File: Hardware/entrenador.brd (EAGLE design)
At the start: 121.9 x 70.8 mm, 68 parts, among them U1 DRV8833

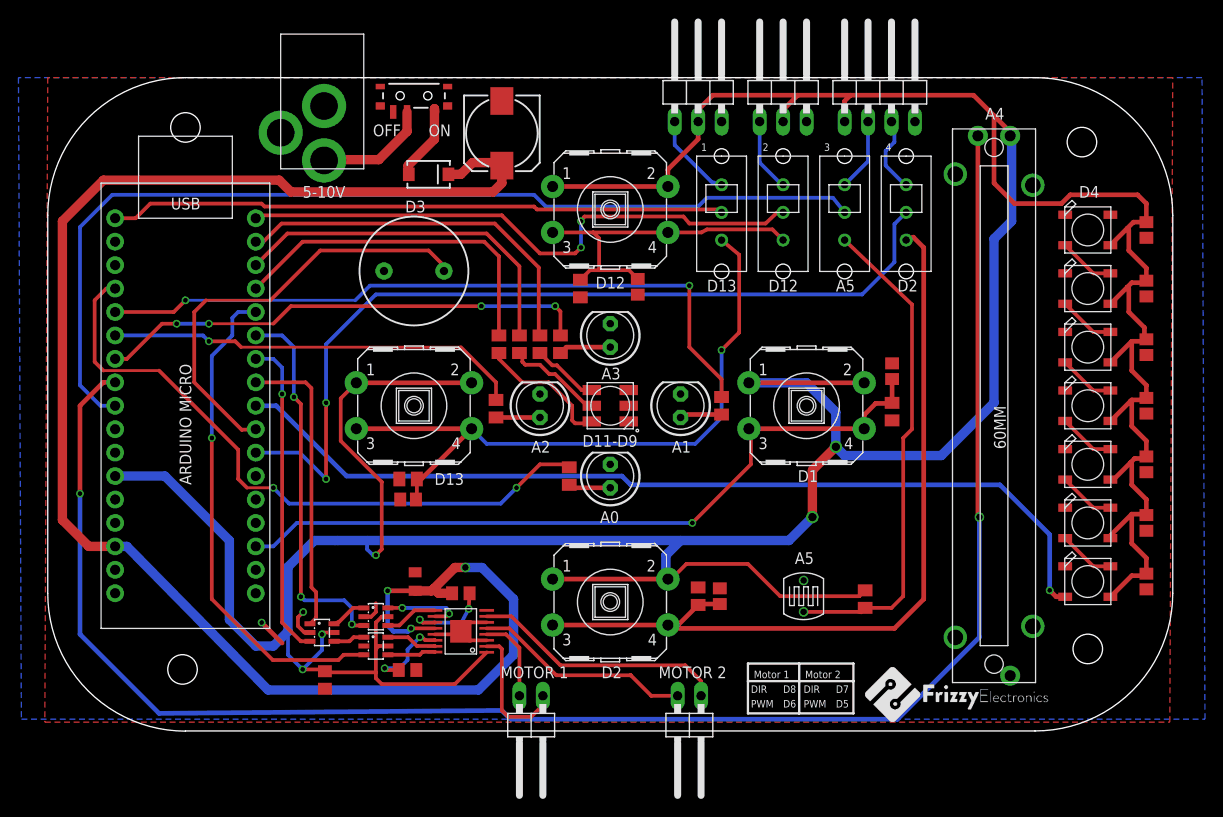
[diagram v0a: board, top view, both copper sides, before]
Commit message: Ultima version
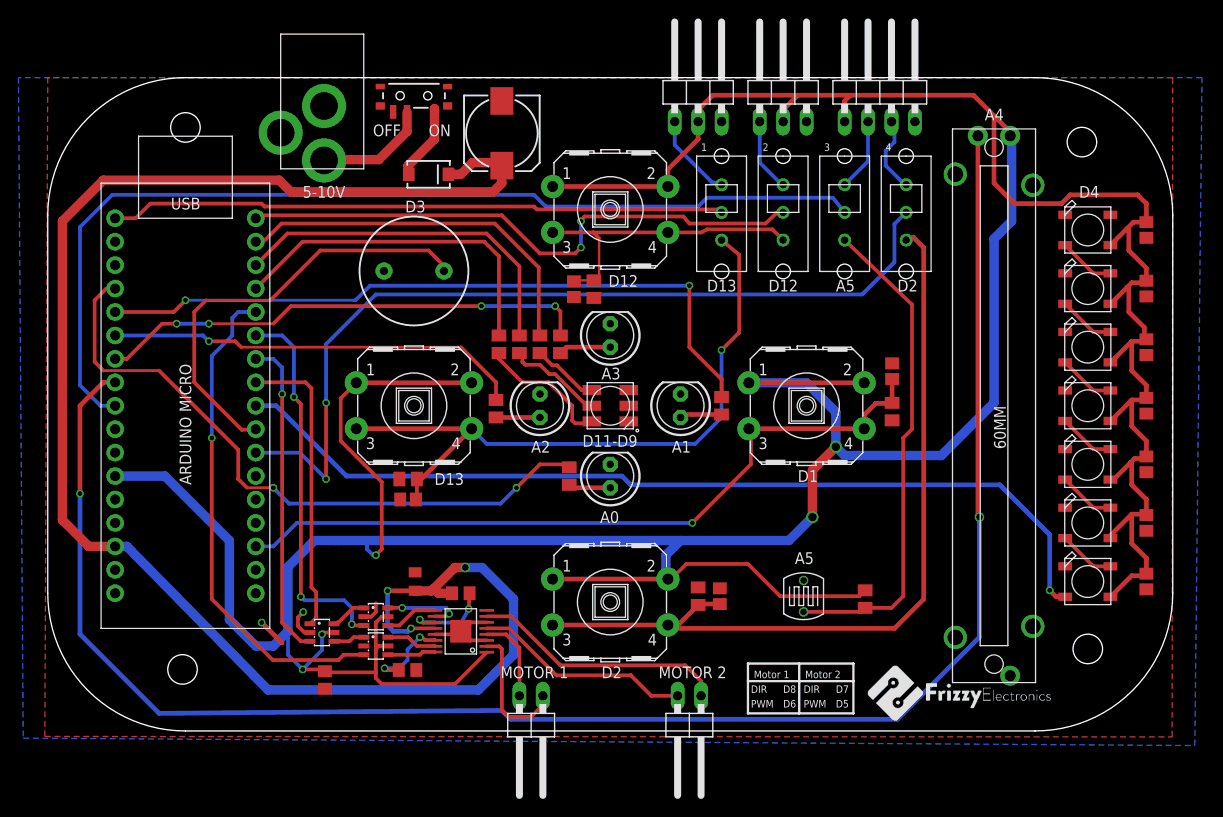
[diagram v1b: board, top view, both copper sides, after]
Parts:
- moved C15 6.93 mm to (57.0, 54.2)
- moved R7 1.46 mm to (59.2, 54.2)
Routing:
- net PB3: track 37.0 -> 33.8 mm
